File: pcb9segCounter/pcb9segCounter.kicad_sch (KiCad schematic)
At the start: 5 parts

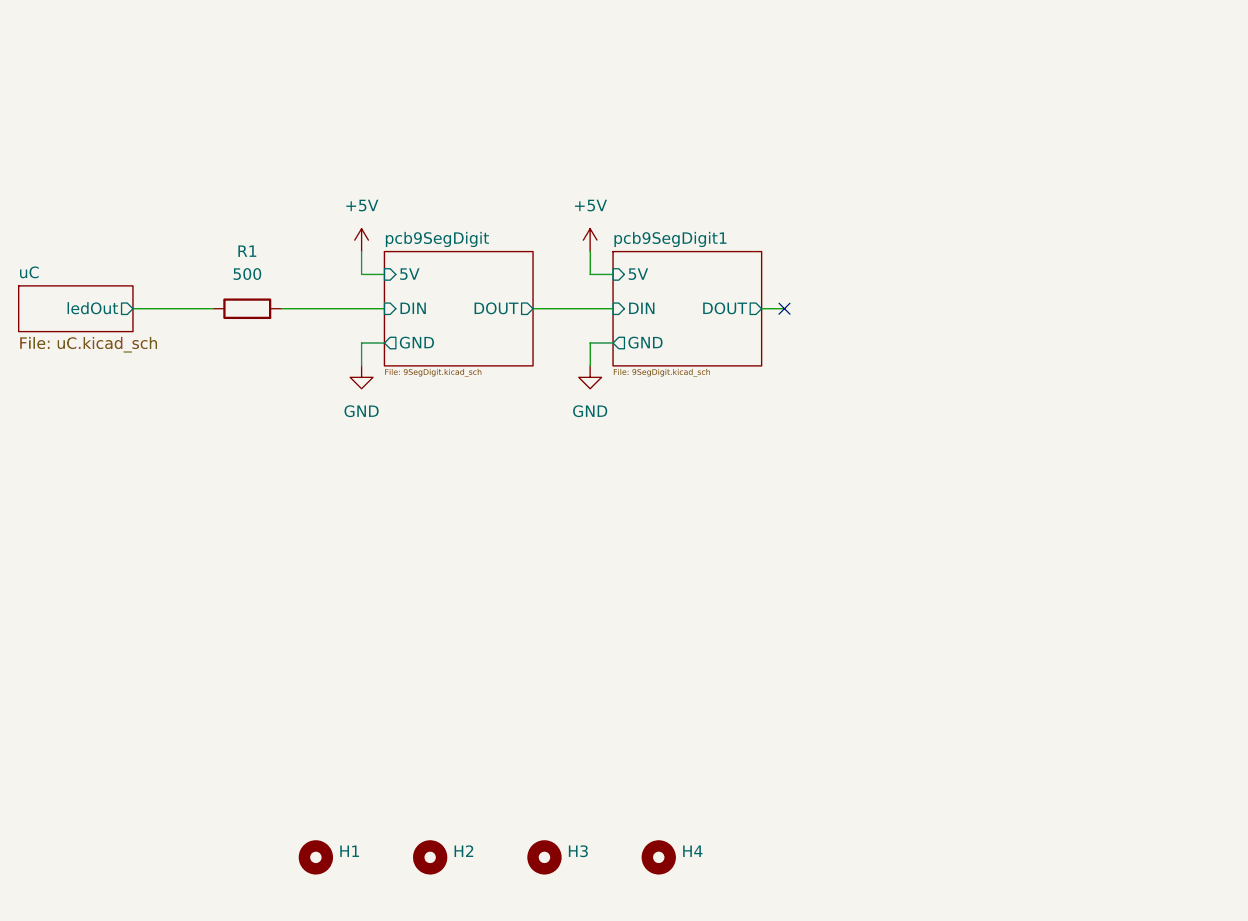
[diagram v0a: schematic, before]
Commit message: Doing lots of cleanup
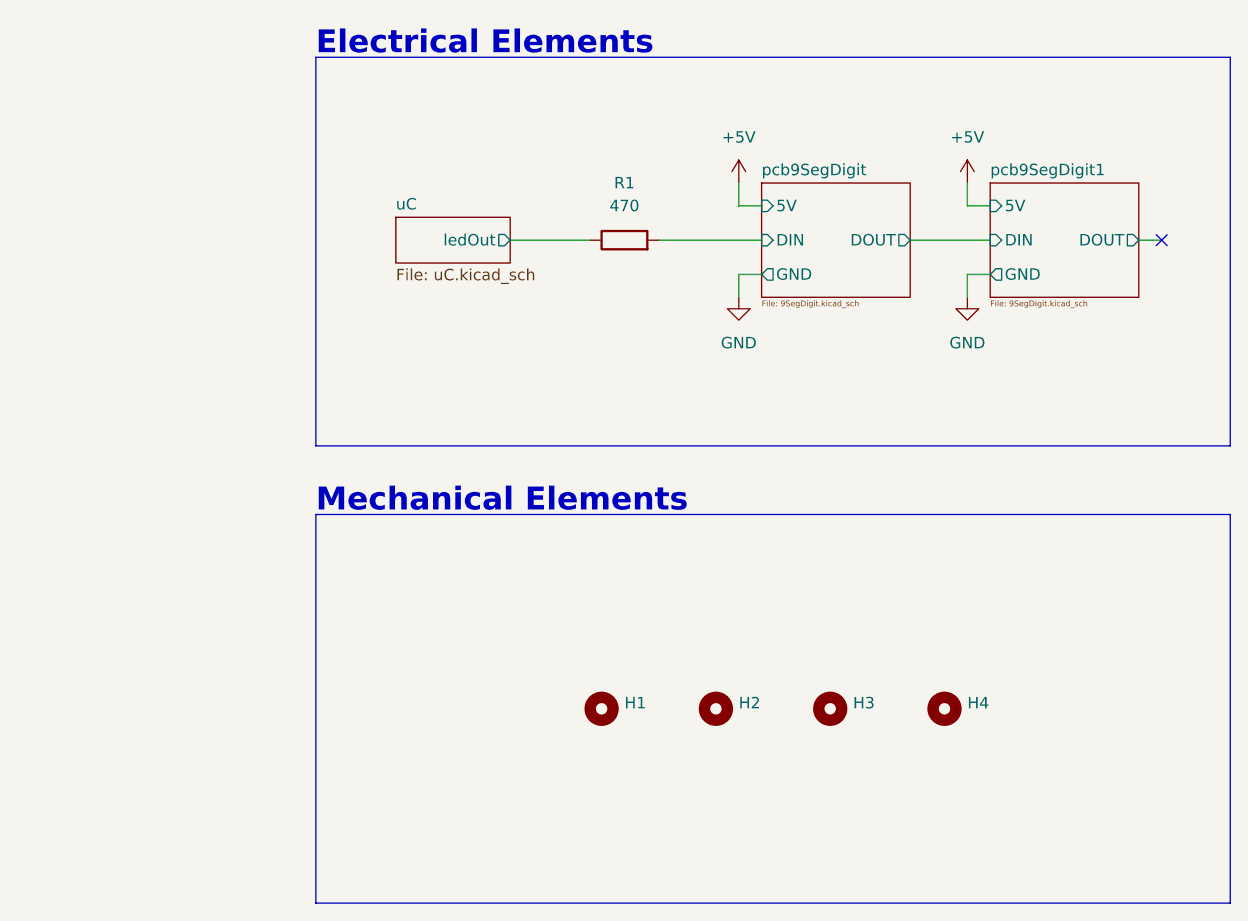
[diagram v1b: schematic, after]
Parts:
- R1: value 500 -> 470
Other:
- note added: "Electrical Elements"
- note added: "Mechanical Elements"
- company: (none) -> Ryan Martin
- title: (none) -> Nine Segment SAO
- moved on the sheet: H1, H2, H3, H4, R1
